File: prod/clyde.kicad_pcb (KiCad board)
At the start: 2 copper layers, 111.4 x 85.7 mm, 26 parts

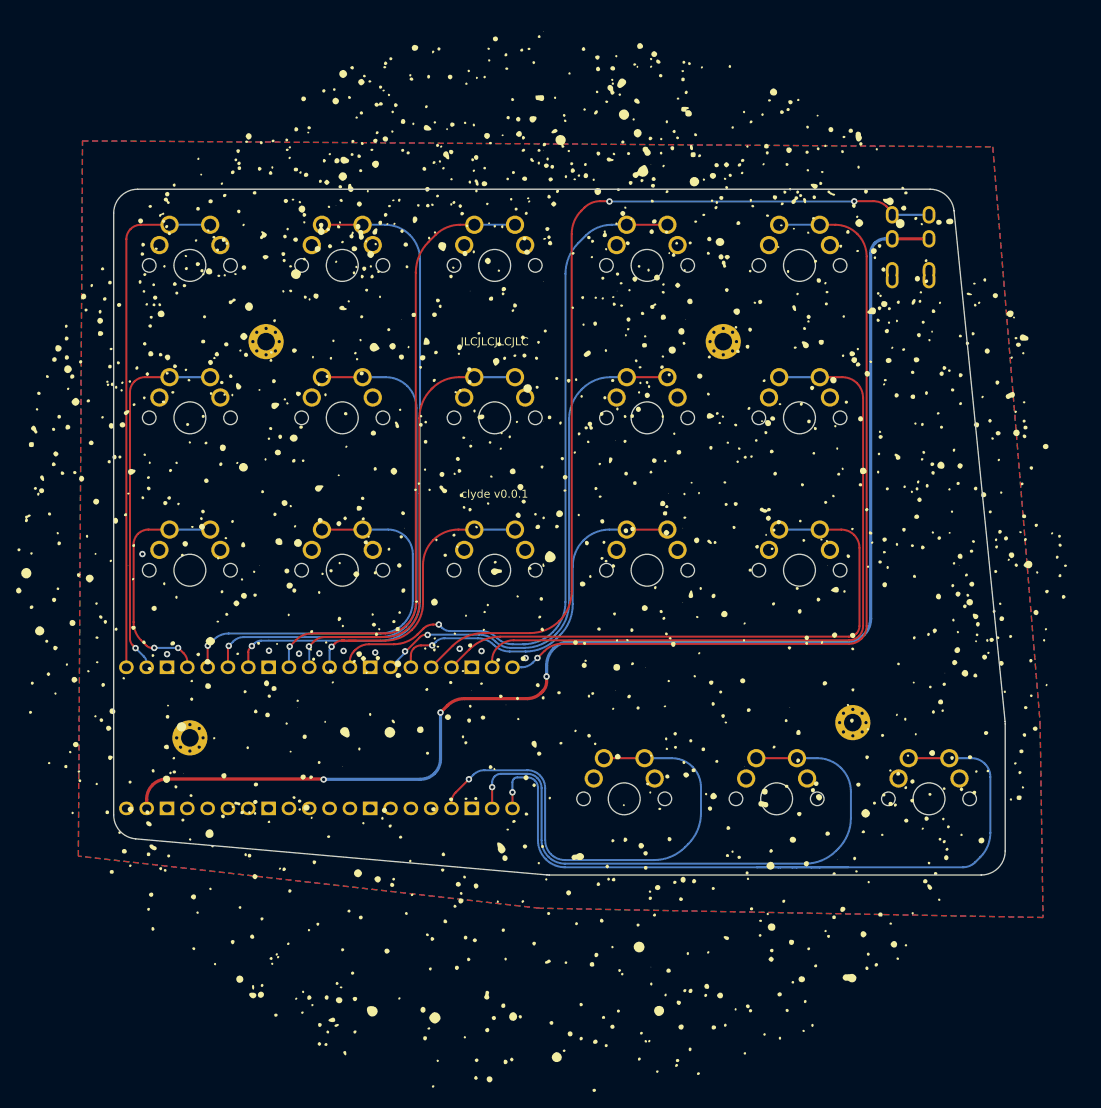
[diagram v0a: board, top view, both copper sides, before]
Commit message: prototypes ordered
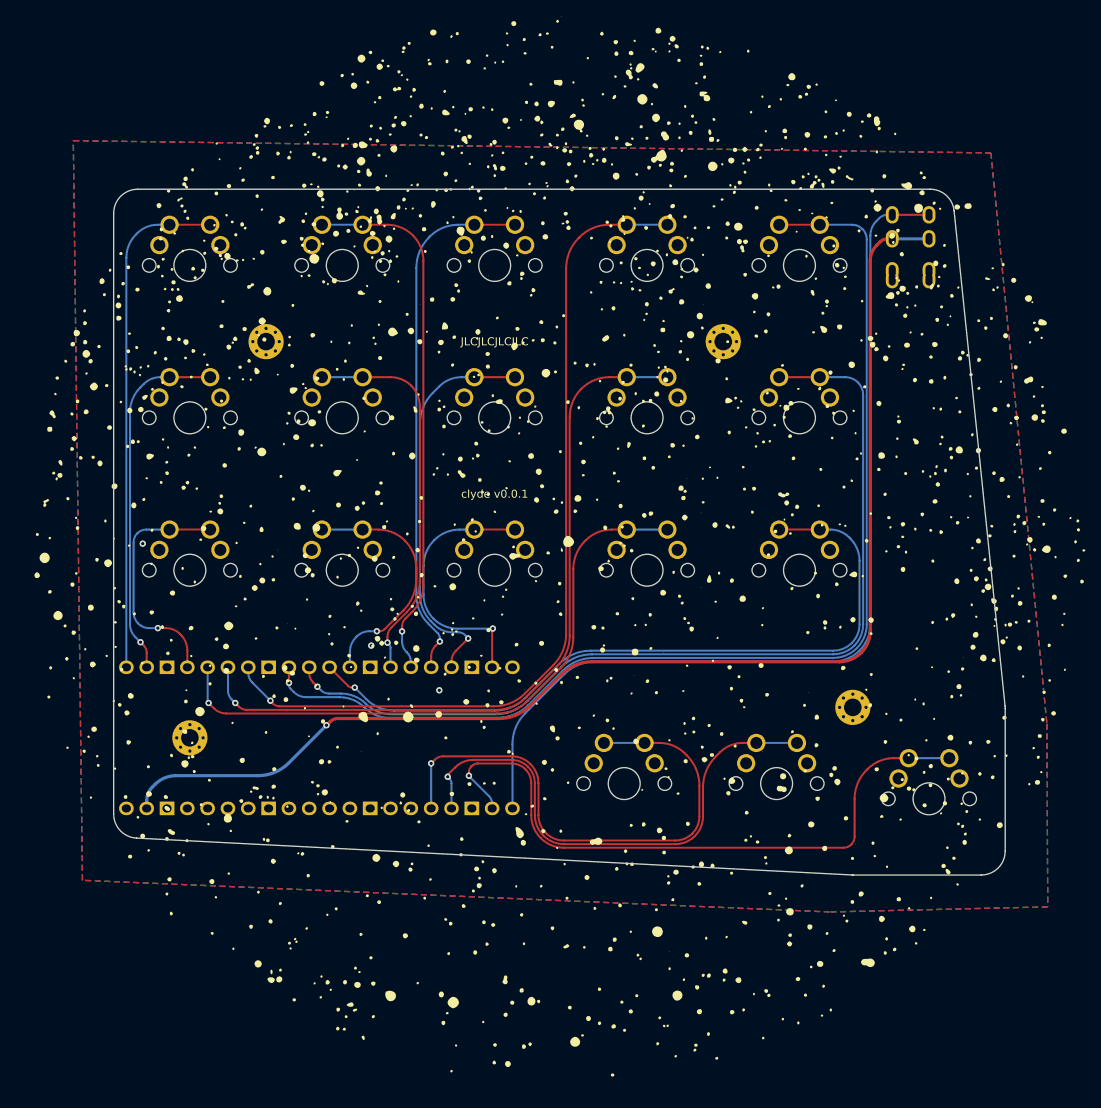
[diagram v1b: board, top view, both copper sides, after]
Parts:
- removed the G*** at (196.5, 151.8)
- removed the G*** at (196.4, 151.3)
- added G***: LOGO, main:north-sky-silk, F.Cu at (198.8, 149.9)
- added G***: LOGO, main:north-sky-silk, B.Cu at (198.8, 149.9)
- moved S16 1.91 mm to (206.7, 179.1)
- moved S17 1.91 mm to (225.7, 179.1)
- moved _4 1.91 mm to (235.3, 169.5)
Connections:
- TRRS1 pad 4: GP12 -> GP16
- U0 pad 10: matrix_middle_home -> matrix_inner_home
- U0 pad 11: matrix_middle_bottom -> matrix_inner_bottom
- U0 pad 12: matrix_index_top -> matrix_ring_bottom
- U0 pad 14: matrix_index_home -> matrix_ring_home
- U0 pad 15: matrix_index_bottom -> matrix_ring_top
- U0 pad 16: GP12 -> matrix_middle_top
- U0 pad 17: matrix_inner_bottom -> matrix_middle_home
- U0 pad 19: matrix_inner_home -> matrix_middle_bottom
- U0 pad 20: matrix_inner_top -> GP15
- U0 pad 21: thumbfan_far_home -> GP16
- U0 pad 22: thumbfan_home_home -> thumbfan_far_home
- U0 pad 24: thumbfan_near_home -> thumbfan_home_home
- U0 pad 25: GP19 -> thumbfan_near_home
- U0 pad 5: matrix_ring_bottom -> matrix_index_bottom
- U0 pad 6: matrix_ring_home -> matrix_index_home
- U0 pad 7: matrix_ring_top -> matrix_index_top
- U0 pad 9: matrix_middle_top -> matrix_inner_top
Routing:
- net GP16: track 0.00 -> 117.3 mm
- net GP12: track 114.2 -> 0.00 mm, vias 2 -> 0
- net matrix_inner_top: track 105.9 -> 140.8 mm
- net matrix_index_bottom: track 45.5 -> 78.3 mm
- net matrix_index_home: track 65.8 -> 93.8 mm, vias 2 -> 1
- net matrix_inner_home: track 90.1 -> 116.3 mm, vias 0 -> 1
- net thumbfan_far_home: track 107.0 -> 81.8 mm
- net matrix_ring_home: track 67.2 -> 48.4 mm
- net matrix_ring_bottom: track 50.1 -> 31.3 mm
- net matrix_inner_bottom: track 74.2 -> 92.9 mm, vias 0 -> 1
- net matrix_ring_top: track 84.2 -> 66.4 mm
- net matrix_index_top: track 90.6 -> 107.7 mm
- net thumbfan_home_home: track 78.5 -> 65.0 mm
- net matrix_middle_top: track 78.1 -> 66.6 mm
- net matrix_middle_home: track 57.2 -> 50.1 mm
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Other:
- outline, holes or cut-outs redrawn

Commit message: layout like split weteor/Kong; outline tweaks
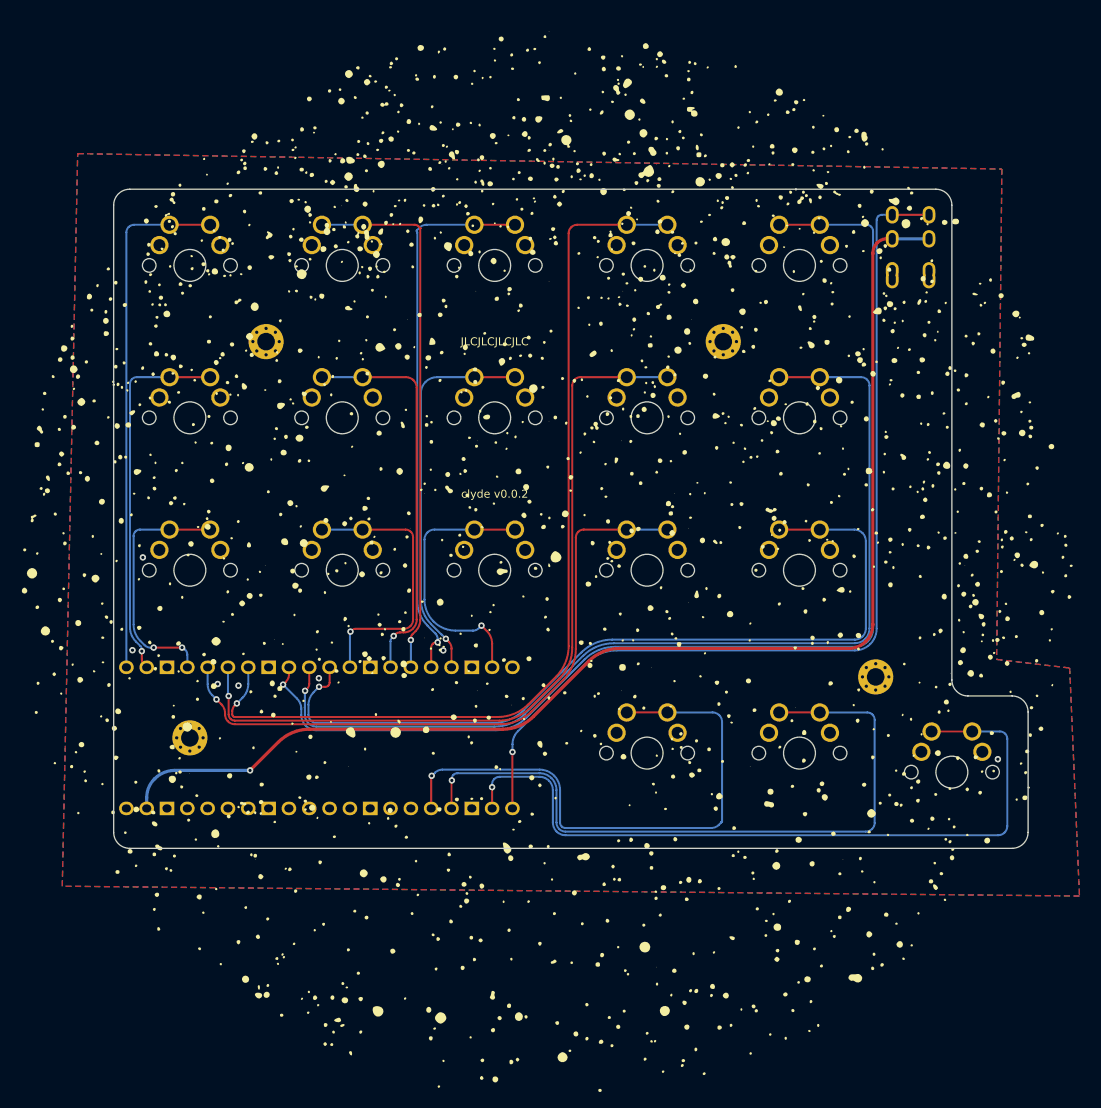
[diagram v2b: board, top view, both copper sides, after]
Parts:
- removed the G*** at (198.8, 149.9) (x2)
- added G***: LOGO, main:north-sky-silk, F.Cu at (197.2, 151.8)
- added G***: LOGO, main:north-sky-silk, B.Cu at (197.0, 151.8)
- moved S16 4.76 mm to (209.6, 175.3)
- moved S17 4.76 mm to (228.6, 175.3)
- moved _4 4.76 mm to (238.1, 165.7)
- moved S18 4.39 mm to (247.7, 177.6)
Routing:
- net thumbfan_home_home: track 65.0 -> 88.8 mm
- net thumbfan_far_home: track 81.8 -> 95.3 mm
- net matrix_inner_bottom: track 92.9 -> 104.9 mm
- net matrix_index_top: track 107.7 -> 117.8 mm
- net matrix_inner_home: track 116.3 -> 124.6 mm
- net matrix_inner_top: track 140.8 -> 146.5 mm
- net matrix_index_home: track 93.8 -> 99.1 mm
- net thumbfan_near_home: track 67.8 -> 71.8 mm
- net matrix_ring_bottom: track 31.3 -> 35.3 mm
- net matrix_index_bottom: track 78.3 -> 81.8 mm
- net matrix_middle_top: track 66.6 -> 68.5 mm
- net matrix_middle_home: track 50.1 -> 48.5 mm
- net matrix_pinky_top: track 64.0 -> 65.4 mm
- net matrix_ring_top: track 66.4 -> 67.7 mm
- net matrix_middle_bottom: track 33.5 -> 34.7 mm
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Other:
- board size 111.4 x 85.7 mm -> 114.3 x 82.4 mm
- board text added: "clyde v0.0.2"
- board text removed: "clyde v0.0.1"
